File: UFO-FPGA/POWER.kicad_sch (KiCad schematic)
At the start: 44 parts, among them J5 USB_B_Micro, Q1 2N7002, U6 PWR convert, U7 PWR convert

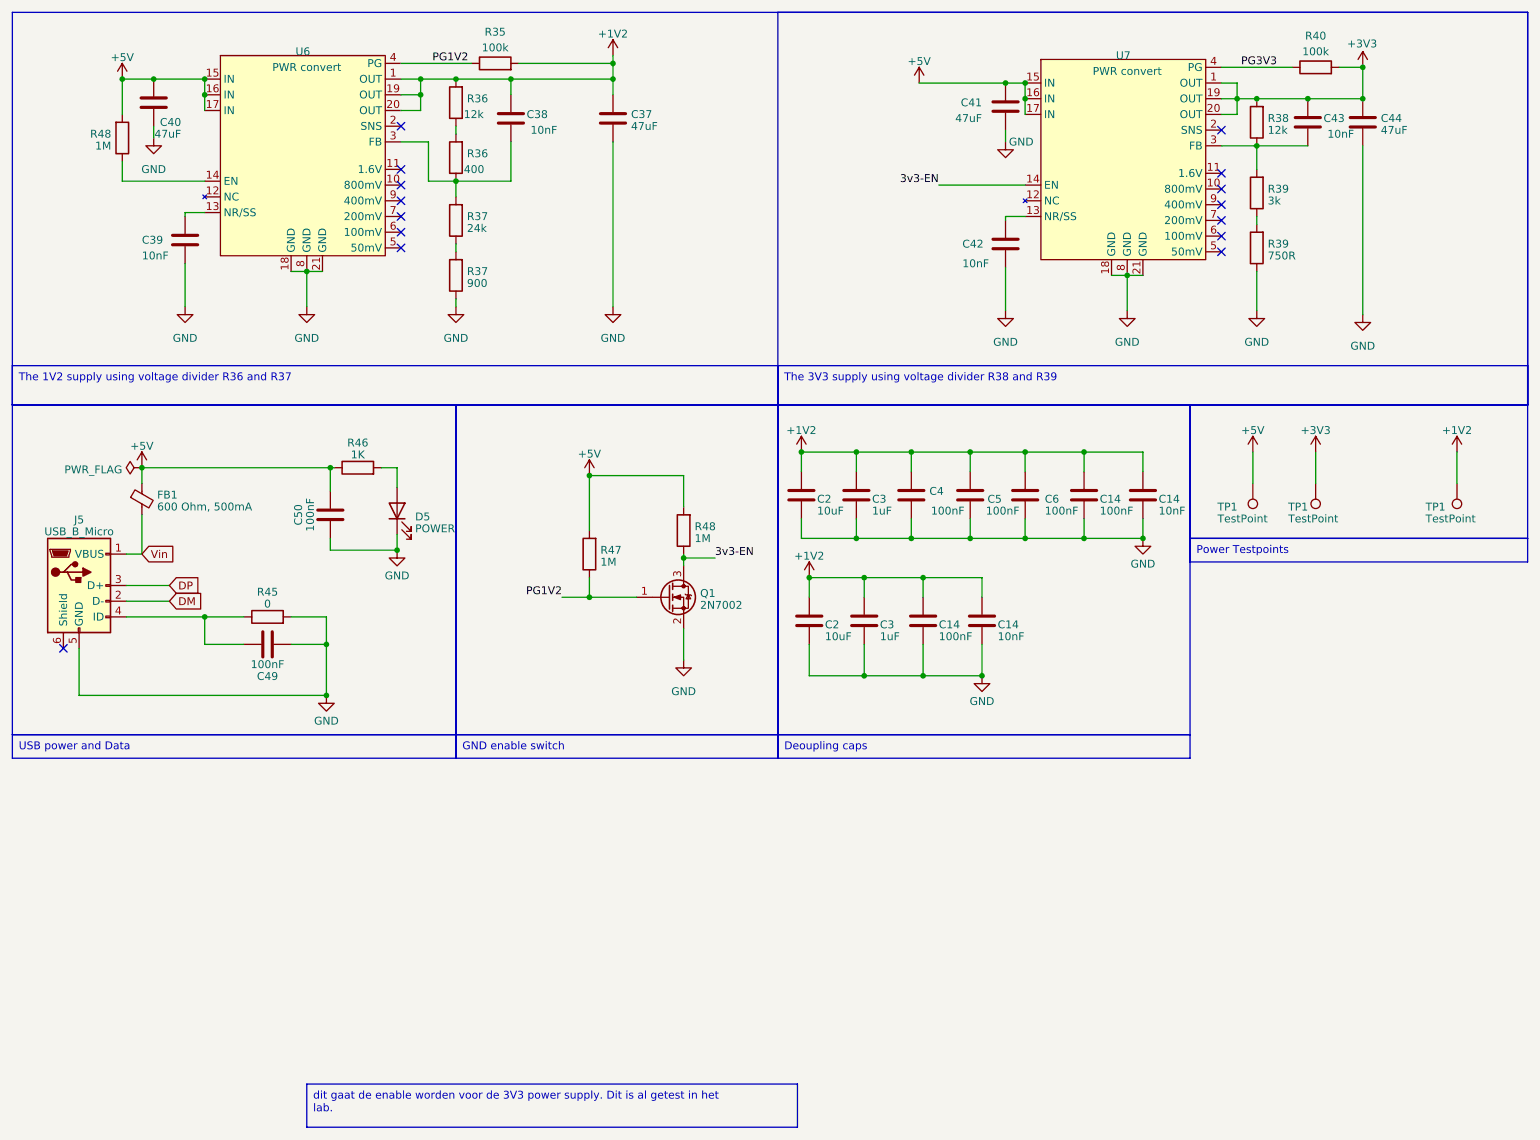
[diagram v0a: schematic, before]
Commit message: PCB
many pcb changes
-started routing
-added vias
-power planes
-ground planes
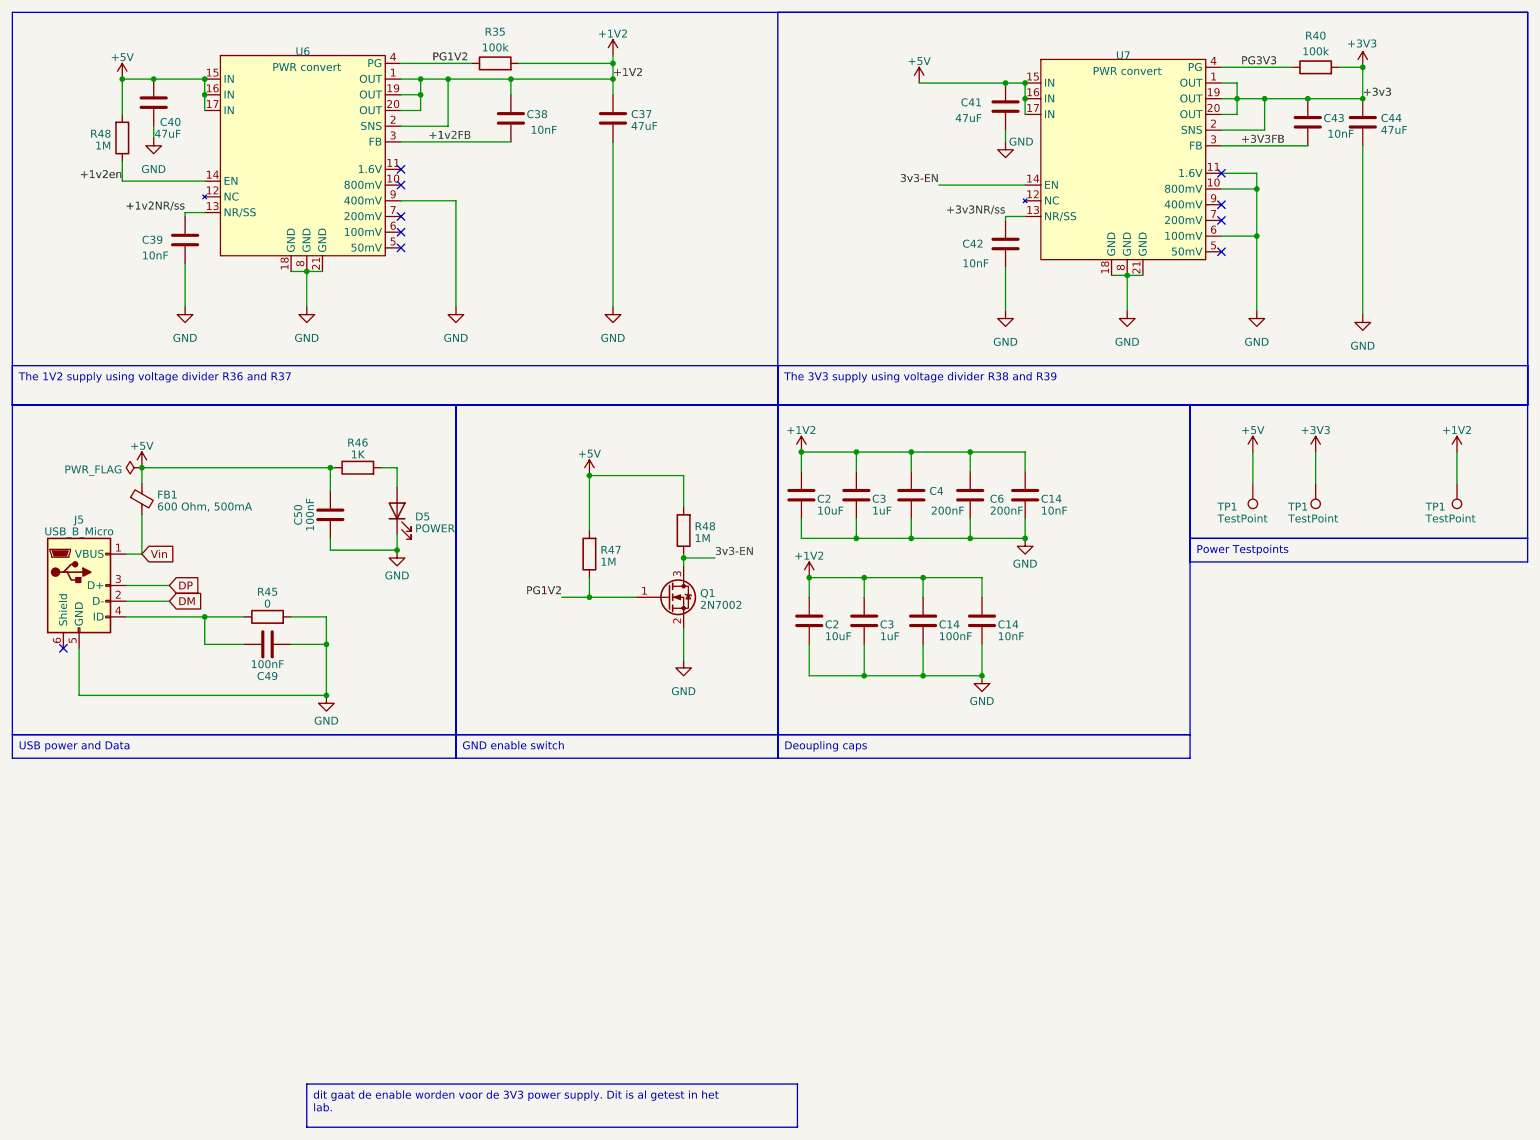
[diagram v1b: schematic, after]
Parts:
- removed C14, C5: 100nF, Capacitor_SMD:C_0805_2012Metric_Pad1.18x1.45mm_HandSolder, symbol Device:C
- removed R36: 400, Resistor_SMD:R_0805_2012Metric_Pad1.20x1.40mm_HandSolder, symbol Device:R
- removed R36: 12k, Resistor_SMD:R_0805_2012Metric_Pad1.20x1.40mm_HandSolder, symbol Device:R
- removed R37: 24k, Resistor_SMD:R_0805_2012Metric_Pad1.20x1.40mm_HandSolder, symbol Device:R
- removed R37: 900, Resistor_SMD:R_0805_2012Metric_Pad1.20x1.40mm_HandSolder, symbol Device:R
- removed R38: 12k, Resistor_SMD:R_0805_2012Metric, symbol Device:R
- removed R39: 750R, Resistor_SMD:R_0805_2012Metric, symbol Device:R
- removed R39: 3k, Resistor_SMD:R_0805_2012Metric, symbol Device:R
- C4, C6: value 100nF -> 200nF
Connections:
- net +1V2: now also U6.2 (SNS)
- net +3V3: now also U7.2 (SNS)
- net GND: now also U6.9 (400mV), U7.10 (800mV), U7.11 (1.6V), U7.6 (100mV)
- net +3V3FB: now reaches C43.2, U7.3 (FB)
- net +1v2NR/ss: now reaches C39.1, U6.13 (NR/SS)
- net +1v2FB: now reaches C38.2, U6.3 (FB)
- net +3v3NR/ss: now reaches C42.1, U7.13 (NR/SS)
- net +1v2en: now reaches R48.1, U6.14 (EN)
- no-connect marks 15 -> 10
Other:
- moved on the sheet: C14, C6

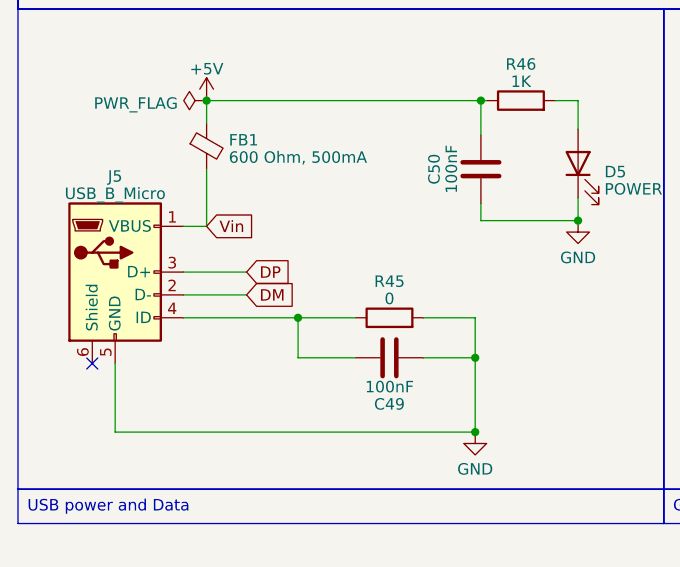
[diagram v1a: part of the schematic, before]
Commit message: pcb prog redesign
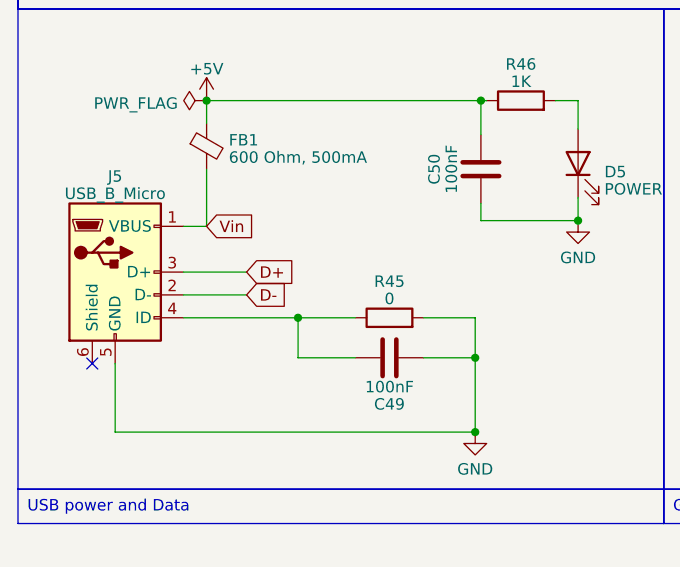
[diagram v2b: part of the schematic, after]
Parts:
- J5: footprint Connector_USB:USB_Micro-AB_Molex_47590-0001 -> Connector_USB:USB_Micro-B_GCT_USB3076-30-A
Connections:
- net DM renamed D-
- net DP renamed D+
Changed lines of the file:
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@@
     (effects (font (size 1.27 1.27)) (justify left bottom))
   )
-  (global_label "DP" (shape input) (at 49.53 107.95 0) (fields_autoplaced)
+  (global_label "D+" (shape input) (at 49.53 107.95 0) (fields_autoplaced)
     (effects (font (size 1.27 1.27)) (justify left))
-    (property "Intersheetrefs" "${INTERSHEET_REFS}" (at 54.9758 107.95 0)
+    (property "Intersheetrefs" "${INTERSHEET_REFS}" (at 55.2782 107.95 0)
       (effects (font (size 1.27 1.27)) (justify left) hide)
     )
@@
     )
   )
-  (global_label "DM" (shape input) (at 49.53 110.49 0) (fields_autoplaced)
+  (global_label "D-" (shape input) (at 49.53 110.49 0) (fields_autoplaced)
     (effects (font (size 1.27 1.27)) (justify left))
-    (property "Intersheetrefs" "${INTERSHEET_REFS}" (at 55.1572 110.49 0)
+    (property "Intersheetrefs" "${INTERSHEET_REFS}" (at 55.2782 110.49 0)
       (effects (font (size 1.27 1.27)) (justify left) hide)
     )
@@
       (effects (font (size 1.27 1.27)))
     )
-    (property "Footprint" "Connector_USB:USB_Micro-AB_Molex_47590-0001" (at 38.735 109.22 0)
-      (effects (font (size 1.27 1.27)) hide)
-    )
+    (property "Footprint" "Connector_USB:USB_Micro-B_GCT_USB3076-30-A" (at 38.735 109.22 0)
+      (effects (font (size 1.27 1.27)) hide)
+    )
